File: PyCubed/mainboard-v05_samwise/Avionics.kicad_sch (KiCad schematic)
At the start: 29 parts, among them SW1 KMR231NG LFS, U1 MAX706RESA, U2 ATSAMD51J20A-AU, Y1 32.768kHz

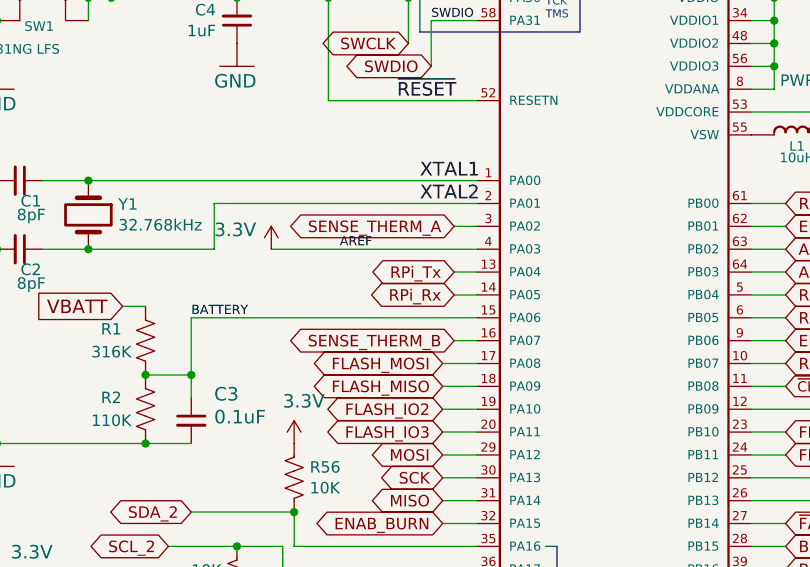
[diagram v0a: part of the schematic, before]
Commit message: made some changes to mainboard
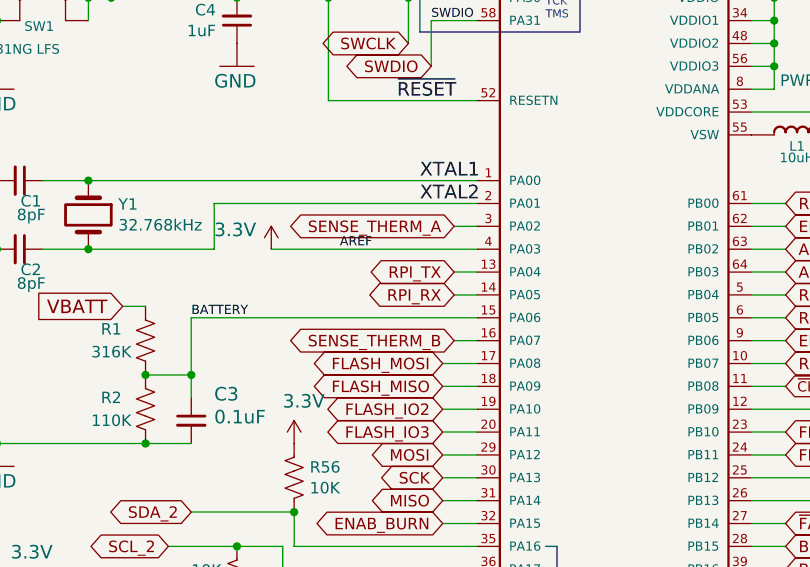
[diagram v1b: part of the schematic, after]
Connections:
- net RPi_Rx renamed RPI_RX
- net RPi_Tx renamed RPI_TX
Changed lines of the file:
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@@
     )
   )
-  (global_label "RPi_Rx" (shape bidirectional) (at 90.17 118.11 180) (fields_autoplaced)
+  (global_label "RPI_RX" (shape bidirectional) (at 90.17 118.11 180) (fields_autoplaced)
     (effects (font (size 1.27 1.27)) (justify right))
-    (property "Intersheetrefs" "${INTERSHEET_REFS}" (at 80.476 118.11 0)
+    (property "Intersheetrefs" "${INTERSHEET_REFS}" (at 80.2946 118.11 0)
       (effects (font (size 1.27 1.27)) (justify right) hide)
     )
@@
     )
   )
-  (global_label "RPi_Tx" (shape bidirectional) (at 90.17 115.57 180) (fields_autoplaced)
+  (global_label "RPI_TX" (shape bidirectional) (at 90.17 115.57 180) (fields_autoplaced)
     (effects (font (size 1.27 1.27)) (justify right))
-    (property "Intersheetrefs" "${INTERSHEET_REFS}" (at 80.7784 115.57 0)
+    (property "Intersheetrefs" "${INTERSHEET_REFS}" (at 80.597 115.57 0)
       (effects (font (size 1.27 1.27)) (justify right) hide)
     )
